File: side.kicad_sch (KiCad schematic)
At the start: 98 parts, among them SW1 SW_Push, SW10 SW_Push, SW11 SW_Push, SW12 SW_Push, SW17 SW_Push, SW18 SW_Push, SW19 SW_Push, SW20 SW_Push, SW25 SW_Push, SW26 SW_Push, SW27 SW_Push, SW28 SW_Push, SW3 SW_Push, SW33 SW_Push, SW34 SW_Push, SW35 SW_Push, SW36 SW_Push, SW41 SW_Push, SW43 RotaryEncoder, SW5 SW_Push, SW7 SW_Push, SW9 SW_Push, U1 XIAO-nRF52840-SMD, U3 PCF8574AP

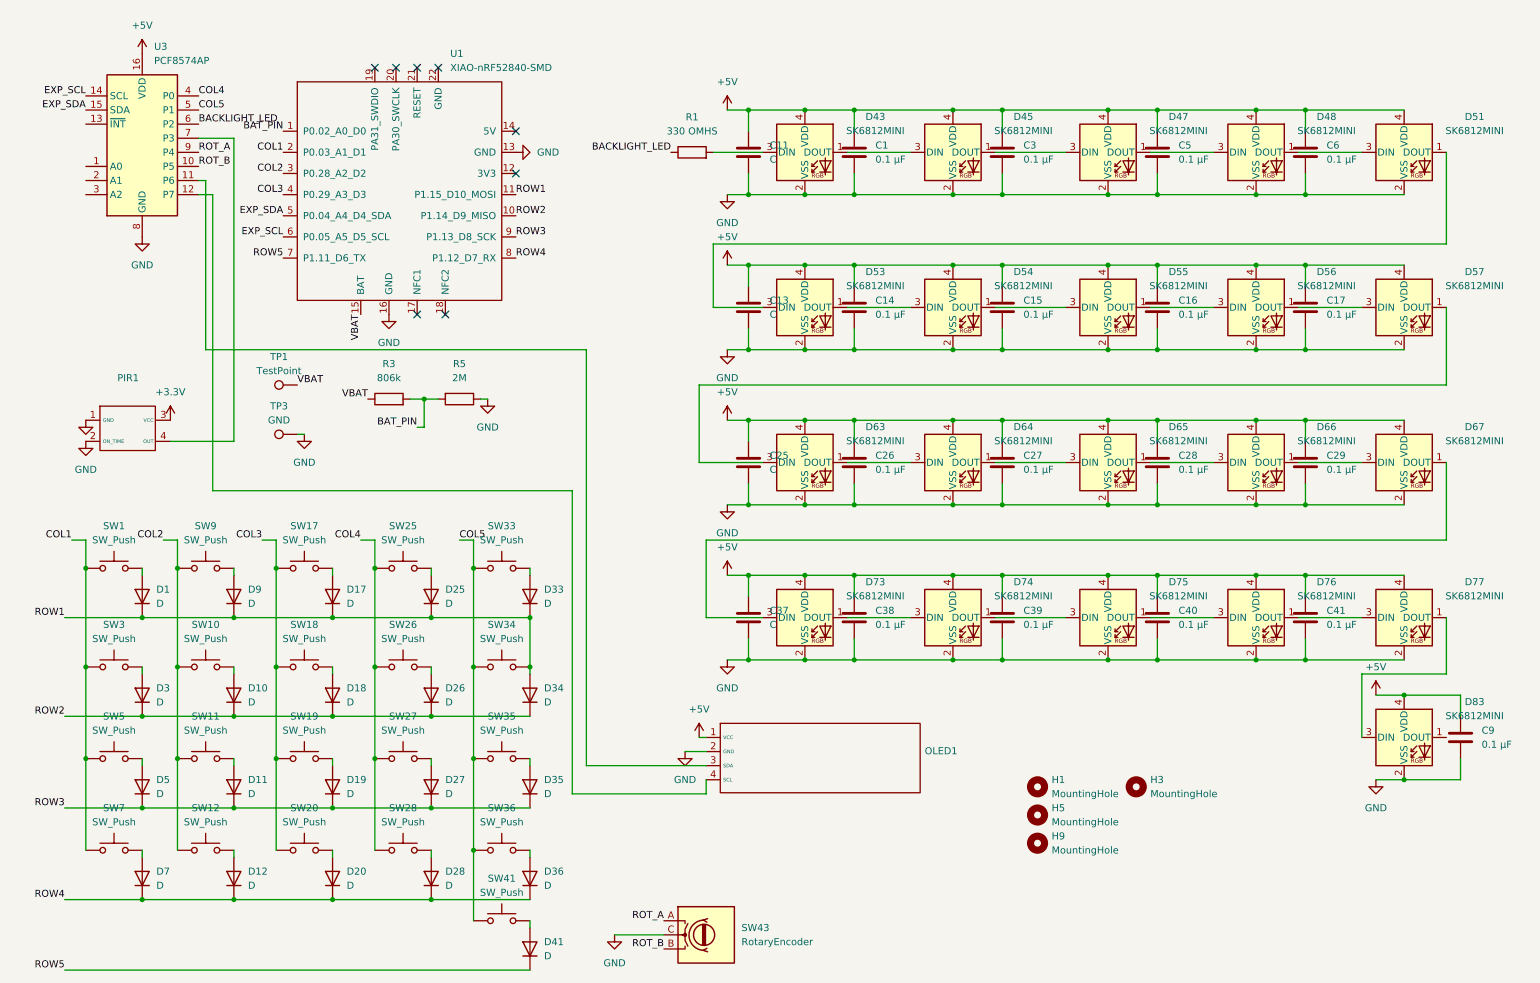
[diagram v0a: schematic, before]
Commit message: done
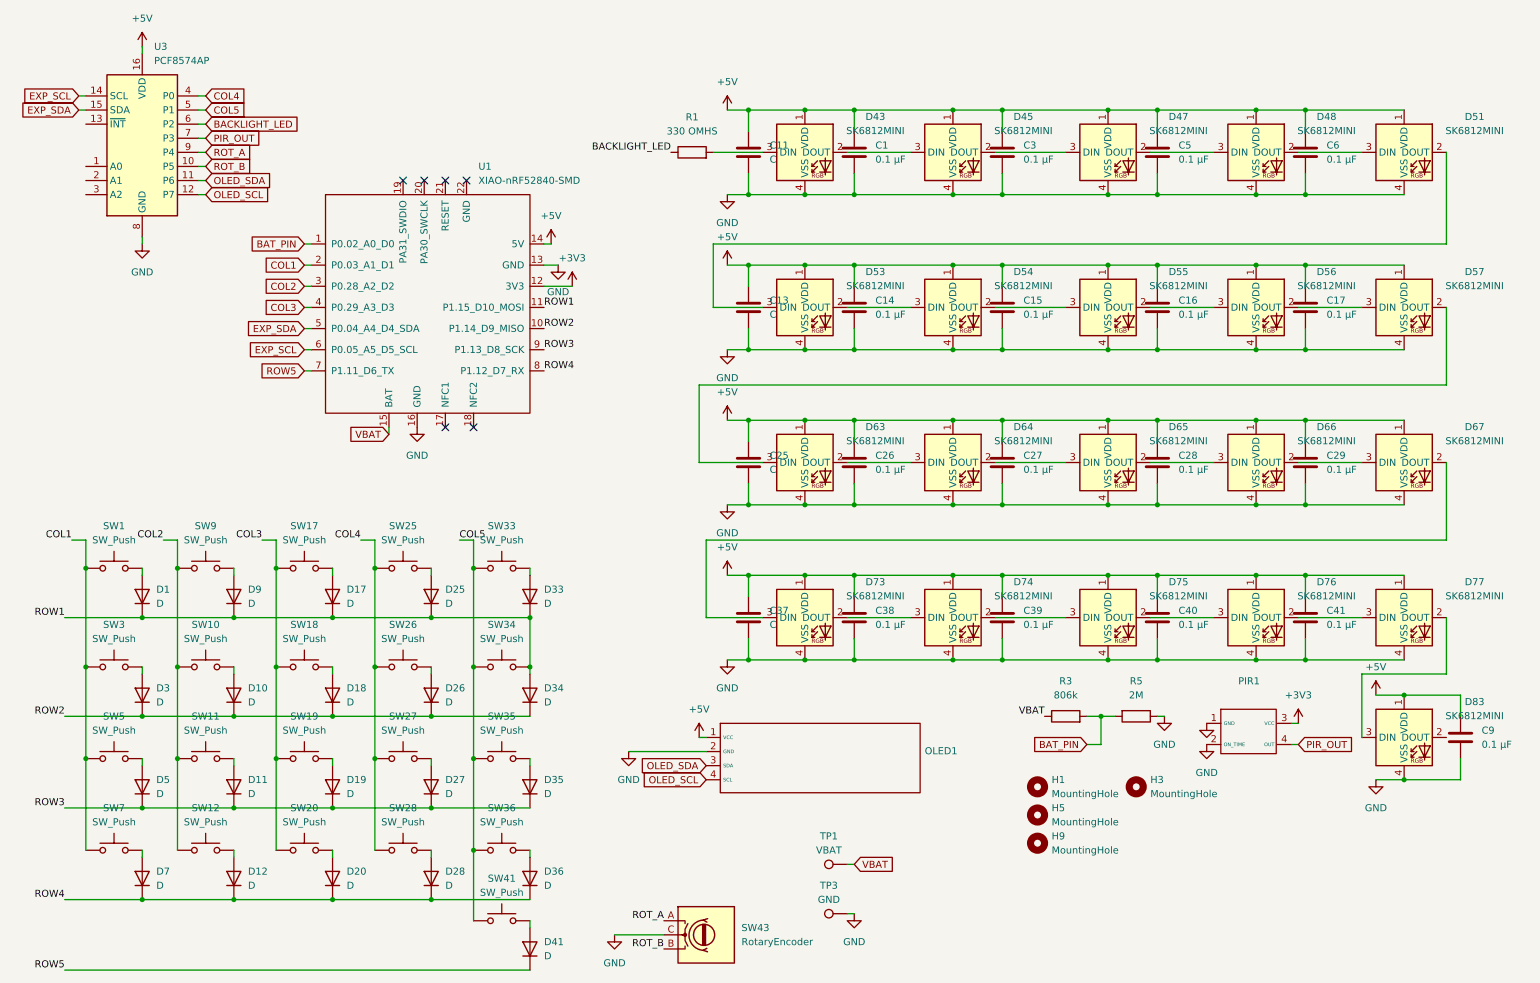
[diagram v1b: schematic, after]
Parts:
- D1, D10, D11, D12, D17, D18, D19, D20, D25, D26, D27, D28, D3, D33, D34, D35, D36, D41, D5, D7, D9: footprint Diode_THT:D_DO-35_SOD27_P7.62mm_Horizontal -> Diode_SMD:D_SOD-123
- D43, D45, D47, D48, D51, D53, D54, D55, D56, D57, D63, D64, D65, D66, D67, D73, D74, D75, D76, D77, D83: footprint LED_SMD:MX_SK6812MINI-E_REV -> PCM_marbastlib-various:LED_6028R; symbol LED:SK6812MINI -> PCM_marbastlib-various:SK6812MINI-E
- OLED1: value ~ -> (none); footprint Display:SSD1306-0.91-OLED-4pin-128x32 -> KiCad-SSD1306-0.91-OLED-4pin-128x32.pretty-master:SSD1306-0.91-OLED-4pin-128x32
- PIR1: value ~ -> (none); footprint Sensor_Motion:BS412 -> BS412:BS412
- SW1, SW10, SW11, SW12, SW17, SW18, SW19, SW20, SW25, SW26, SW27, SW28, SW3, SW33, SW34, SW35, SW36, SW41, SW5, SW9: footprint PCM_marbastlib-mx:SW_MX_1u -> marbastlib-choc:SW_choc_v1_HS_CPG135001S30_1u
- SW7: footprint PCM_marbastlib-mx:SW_MX_1u -> marbastlib-choc:SW_choc_v1_HS_CPG135001S30_1.5u
- TP1: value TestPoint -> VBAT
- U1: footprint RF_WiFi:modified-XIAO-nRF52840-SMD -> modified-xiao:modified-XIAO-nRF52840-SMD
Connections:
- net +3.3V is gone; now on net +3V3: PIR1.3 (VCC)
- net +5V: now also D43.1 (VDD), D45.1 (VDD), D47.1 (VDD), D48.1 (VDD), D51.1 (VDD), D53.1 (VDD), D54.1 (VDD), D55.1 (VDD), D56.1 (VDD), D57.1 (VDD), D63.1 (VDD), D64.1 (VDD), D65.1 (VDD), D66.1 (VDD), D67.1 (VDD), D73.1 (VDD), D74.1 (VDD), D75.1 (VDD), D76.1 (VDD), D77.1 (VDD), D83.1 (VDD), U1.14 (5V); no longer D43.4 (VDD), D45.4 (VDD), D47.4 (VDD), D48.4 (VDD), D51.4 (VDD), D53.4 (VDD), D54.4 (VDD), D55.4 (VDD), D56.4 (VDD), D57.4 (VDD), D63.4 (VDD), D64.4 (VDD), D65.4 (VDD), D66.4 (VDD), D67.4 (VDD), D73.4 (VDD), D74.4 (VDD), D75.4 (VDD), D76.4 (VDD), D77.4 (VDD), D83.4 (VDD)
- net GND: now also D43.4 (VSS), D45.4 (VSS), D47.4 (VSS), D48.4 (VSS), D51.4 (VSS), D53.4 (VSS), D54.4 (VSS), D55.4 (VSS), D56.4 (VSS), D57.4 (VSS), D63.4 (VSS), D64.4 (VSS), D65.4 (VSS), D66.4 (VSS), D67.4 (VSS), D73.4 (VSS), D74.4 (VSS), D75.4 (VSS), D76.4 (VSS), D77.4 (VSS), D83.4 (VSS); no longer D43.2 (VSS), D45.2 (VSS), D47.2 (VSS), D48.2 (VSS), D51.2 (VSS), D53.2 (VSS), D54.2 (VSS), D55.2 (VSS), D56.2 (VSS), D57.2 (VSS), D63.2 (VSS), D64.2 (VSS), D65.2 (VSS), D66.2 (VSS), D67.2 (VSS), D73.2 (VSS), D74.2 (VSS), D75.2 (VSS), D76.2 (VSS), D77.2 (VSS), D83.2 (VSS)
- net +3V3: now reaches U1.12 (3V3)
- net OLED_SDA: now reaches OLED1.3 (SDA), U3.11 (P6)
- net OLED_SCL: now reaches OLED1.4 (SCL), U3.12 (P7)
- net PIR_OUT: now reaches PIR1.4 (OUT), U3.7 (P3)
- net at D47.3 (DIN): now also D45.2 (DOUT); no longer D45.1 (DOUT)
- net at D45.3 (DIN): now also D43.2 (DOUT); no longer D43.1 (DOUT)
- net at D53.3 (DIN): now also D51.2 (DOUT); no longer D51.1 (DOUT)
- net at D51.3 (DIN): now also D48.2 (DOUT); no longer D48.1 (DOUT)
- net at D75.3 (DIN): now also D74.2 (DOUT); no longer D74.1 (DOUT)
- net at D74.3 (DIN): now also D73.2 (DOUT); no longer D73.1 (DOUT)
- net at D54.3 (DIN): now also D53.2 (DOUT); no longer D53.1 (DOUT)
- net at D73.3 (DIN): now also D67.2 (DOUT); no longer D67.1 (DOUT)
- net at D67.3 (DIN): now also D66.2 (DOUT); no longer D66.1 (DOUT)
- net at D55.3 (DIN): now also D54.2 (DOUT); no longer D54.1 (DOUT)
- net at D65.3 (DIN): now also D64.2 (DOUT); no longer D64.1 (DOUT)
- net at D64.3 (DIN): now also D63.2 (DOUT); no longer D63.1 (DOUT)
- net at D56.3 (DIN): now also D55.2 (DOUT); no longer D55.1 (DOUT)
- net at D63.3 (DIN): now also D57.2 (DOUT); no longer D57.1 (DOUT)
- net at D48.3 (DIN): now also D47.2 (DOUT); no longer D47.1 (DOUT)
- net at D57.3 (DIN): now also D56.2 (DOUT); no longer D56.1 (DOUT)
- net at D76.3 (DIN): now also D75.2 (DOUT); no longer D75.1 (DOUT)
- net at D83.3 (DIN): now also D77.2 (DOUT); no longer D77.1 (DOUT)
- net at D66.3 (DIN): now also D65.2 (DOUT); no longer D65.1 (DOUT)
- net at D77.3 (DIN): now also D76.2 (DOUT); no longer D76.1 (DOUT)
- no-connect marks 8 -> 6
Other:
- moved on the sheet: PIR1, R3, R5, U1

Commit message: fdhshfadshkfdsahhfadshjkfds
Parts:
- R1: footprint Resistor_THT:R_Axial_DIN0207_L6.3mm_D2.5mm_P10.16mm_Horizontal -> Resistor_THT:R_Axial_DIN0207_L6.3mm_D2.5mm_P7.62mm_Horizontal
- R3, R5: footprint Resistor_THT:R_Axial_DIN0207_L6.3mm_D2.5mm_P10.16mm_Horizontal -> Resistor_SMD:R_0805_2012Metric
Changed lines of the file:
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@@
 			)
 		)
-		(property "Footprint" "Resistor_THT:R_Axial_DIN0207_L6.3mm_D2.5mm_P10.16mm_Horizontal"
+		(property "Footprint" "Resistor_SMD:R_0805_2012Metric"
 			(at 199.39 135.128 90)
 			(hide yes)
@@
 			)
 		)
-		(property "Footprint" "Resistor_THT:R_Axial_DIN0207_L6.3mm_D2.5mm_P10.16mm_Horizontal"
+		(property "Footprint" "Resistor_THT:R_Axial_DIN0207_L6.3mm_D2.5mm_P7.62mm_Horizontal"
 			(at 132.08 33.528 90)
 			(hide yes)
@@
 			)
 		)
-		(property "Footprint" "Resistor_THT:R_Axial_DIN0207_L6.3mm_D2.5mm_P10.16mm_Horizontal"
+		(property "Footprint" "Resistor_SMD:R_0805_2012Metric"
 			(at 212.09 131.572 90)
 			(hide yes)
